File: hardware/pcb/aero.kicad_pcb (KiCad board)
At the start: 4 copper layers, 39.1 x 46.2 mm, 91 parts, among them CON1 USB-MICRO-B, CON2 MMCX_CONN, J1 CORTEX_DBG_CONN, J2 LiPoly_Conn, Q1 Q_NPN_BEC, SW1 SW_PUSH, U1 STM32L151C8, U2 nRF8001, U3 ms5611, U4 BMX055, U5 AT45DB321E, U6 BQ24040DSQ, U7 TPS783, U8 TPS61041, U9 ZXMHC6A07N8, Y1 Crystal, Y2 Crystal, Y3 32.768KHz, Y4 16MHz

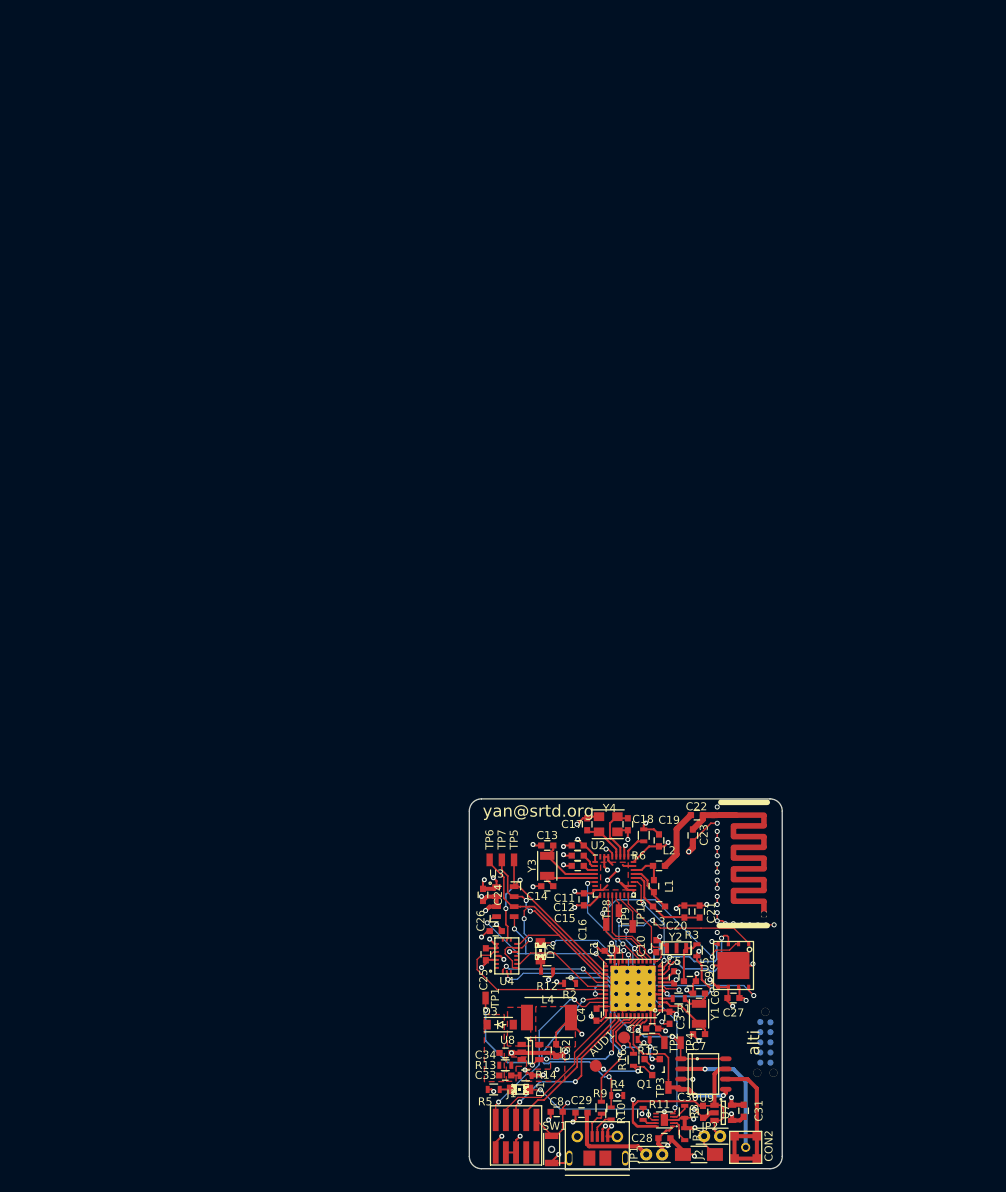
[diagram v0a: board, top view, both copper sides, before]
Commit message: more progress on new layout
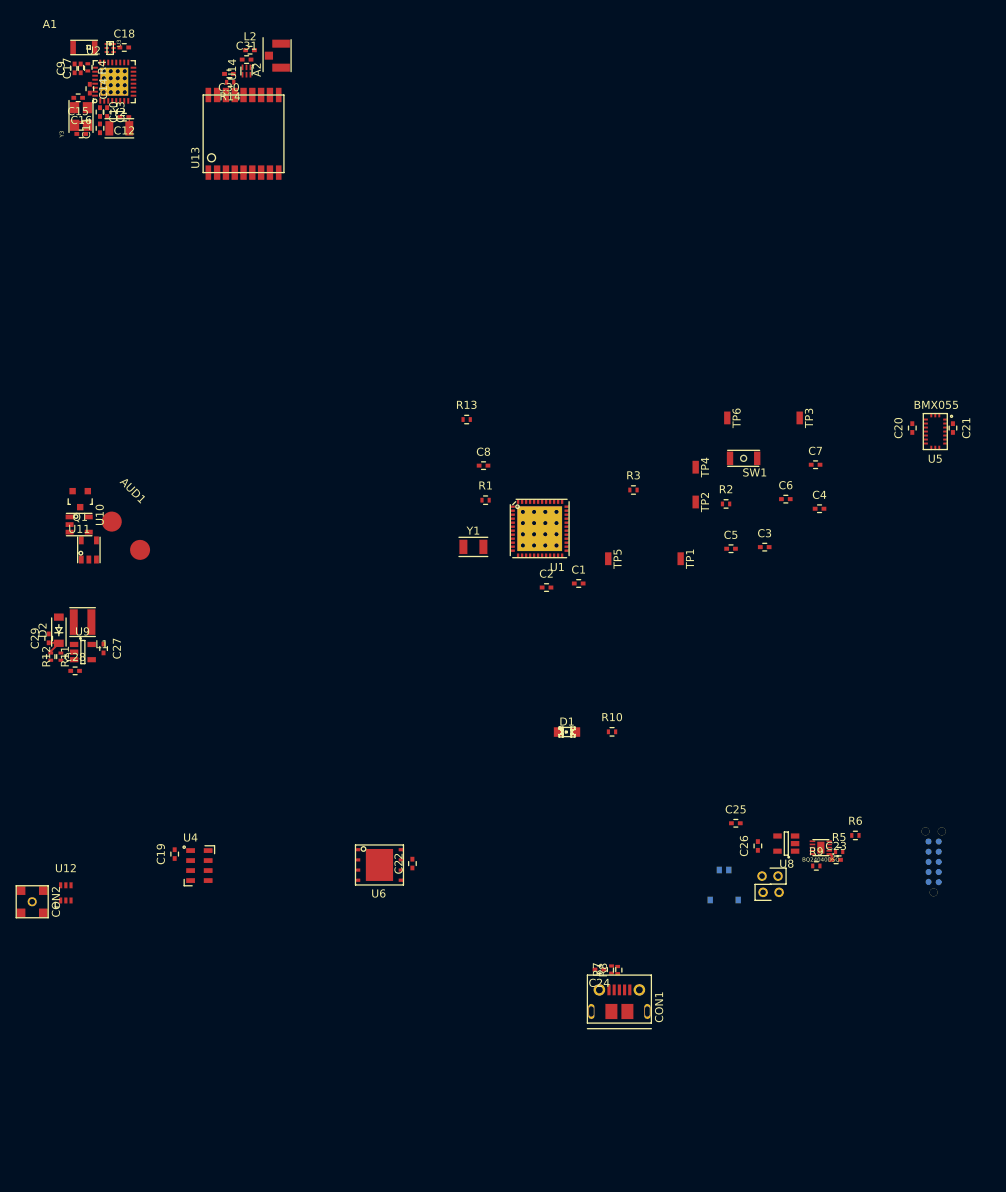
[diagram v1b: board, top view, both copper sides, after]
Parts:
- removed Ant_Bluetooth: VAL**, aero:Ant_Bluetooth
- removed C32: 4.7uF, Capacitors_SMD:C_0603
- removed C33: 22pF, Capacitors_SMD:C_0603
- removed C34: 100nF, Capacitors_SMD:C_0603
- removed D3: D_Schottky, Diodes_SMD:SOD-123
- removed L3: 5.6nH, Capacitors_SMD:C_0603
- removed L4: 10u, aero:SDR0703
- removed R15: 3k, Resistors_SMD:R_0603
- removed R16: 2k, Resistors_SMD:R_0603
- removed REF**: TC2050-IDC-NL, aero:TC2050-IDC-NL
- removed TP10, TP7, TP8, TP9: Test_Point, aero:TP_0603
- removed Y4: 16MHz, aero:crystal_SMD_3225
- added A1: 2450AT18A100, aero:2450AT18A100, F.Cu at (112.3, 17.8)
- added A2: U.FL_Antenna, aero:U.FL, F.Cu at (137.0, 18.9)
- added U10: BU4SU69G2, aero:SSOP-5, F.Cu at (111.8, 77.5)
- added U11: BU4SU69G2, aero:SSOP-5, F.Cu at (113.0, 80.6)
- added U12: NC7WZ17, Housings_SOT-23_SOT-143_TSOT-6:SC-70-6, F.Cu at (110.1, 123.5)
- added U13: u-blox_max-7c/q, aero:ublox_MAX7, F.Cu at (132.3, 28.6)
- added U14: MAX2659, aero:6-µDFN, F.Cu at (132.7, 20.8)
- C1, C2, C3, C4, C5, C6, C7, C8: footprint Capacitors_SMD:C_0603 -> Capacitors_SMD:C_0402
- C10, C14, C9: value 15pF -> 100nF; footprint Capacitors_SMD:C_0603 -> Capacitors_SMD:C_0402
- C11, C12: value 100nF -> 15pF; footprint Capacitors_SMD:C_0603 -> Capacitors_SMD:C_0402
- C13: value 15pF -> 33nF; footprint Capacitors_SMD:C_0603 -> Capacitors_SMD:C_0402
- C15: value 33nF -> 12pF; footprint Capacitors_SMD:C_0603 -> Capacitors_SMD:C_0402
- C16: value 100nF -> 12pF; footprint Capacitors_SMD:C_0603 -> Capacitors_SMD:C_0402
- C17: value 12pF -> 1.0nF; footprint Capacitors_SMD:C_0603 -> Capacitors_SMD:C_0402
- C18: value 12pF -> 2.2nF; footprint Capacitors_SMD:C_0603 -> Capacitors_SMD:C_0402
- C19: value 1.0nF -> 100nF; footprint Capacitors_SMD:C_0603 -> Capacitors_SMD:C_0402
- C20: value 2.2nF -> 100nF; footprint Capacitors_SMD:C_0603 -> Capacitors_SMD:C_0402
- C21: value NC -> 100nF; footprint Capacitors_SMD:C_0603 -> Capacitors_SMD:C_0402
- C22: value 1.8pF -> 100nF; footprint Capacitors_SMD:C_0603 -> Capacitors_SMD:C_0402
- C23: value 1.2pF -> 1uF; footprint Capacitors_SMD:C_0603 -> Capacitors_SMD:C_0402
- C24, C25: value 100nF -> 1uF; footprint Capacitors_SMD:C_0603 -> Capacitors_SMD:C_0402
- C26: value 100nF -> 2.2uF; footprint Capacitors_SMD:C_0603 -> Capacitors_SMD:C_0402
- C27: value 100nF -> 4.7uF; footprint Capacitors_SMD:C_0603 -> Capacitors_SMD:C_0402
- C28: value 1uF -> 22pF; footprint Capacitors_SMD:C_0603 -> Capacitors_SMD:C_0402
- C29: value 1uF -> 100nF; footprint Capacitors_SMD:C_0603 -> Capacitors_SMD:C_0402
- C30: value 1uF -> 33nF; footprint Capacitors_SMD:C_0603 -> Capacitors_SMD:C_0402
- C31: value 2.2uF -> 470pF; footprint Capacitors_SMD:C_0603 -> Capacitors_SMD:C_0402
- D2: value LED -> D_Schottky; footprint LEDs:LED-0805 -> Diodes_SMD:SOD-123
- J1: footprint aero:FTSH-105-01 -> aero:TC2050-IDC-NL; moved to B.Cu
- J2: footprint Capacitors_SMD:C_1206_HandSoldering -> aero:Conn_Molex_78171-02; moved to B.Cu
- JP1, JP2: footprint aero:Pin_Header_1x02 -> aero:Pin_Header_1x02_2mm
- L1: value 8.2nH -> 10u; footprint Capacitors_SMD:C_0603 -> aero:IND-744029100
- L2: value 3.9nH -> 6.8nH; footprint Capacitors_SMD:C_0603 -> Capacitors_SMD:C_0402
- Q1: value Q_NPN_BEC -> BSS138
- R1, R2: footprint Resistors_SMD:R_0603 -> Resistors_SMD:R_0402
- R10: value 22 -> 200; footprint Resistors_SMD:R_0603 -> Resistors_SMD:R_0402
- R11: value 10k -> 2.21m; footprint Resistors_SMD:R_0603 -> Resistors_SMD:R_0402
- R12: value 120 -> 309k; footprint Resistors_SMD:R_0603 -> Resistors_SMD:R_0402
- R13: value 2.21m -> 30k; footprint Resistors_SMD:R_0603 -> Resistors_SMD:R_0402
- R14: value 140k -> 10k; footprint Resistors_SMD:R_0603 -> Resistors_SMD:R_0402
- R3: value 220 -> 1.5k; footprint Resistors_SMD:R_0603 -> Resistors_SMD:R_0402
- R4: value 1.5k -> 22k; footprint Resistors_SMD:R_0603 -> Resistors_SMD:R_0402
- R5: value 1.5k -> 825; footprint Resistors_SMD:R_0603 -> Resistors_SMD:R_0402
- R6: value 22k -> 2k; footprint Resistors_SMD:R_0603 -> Resistors_SMD:R_0402
- R7: value 825 -> 22; footprint Resistors_SMD:R_0603 -> Resistors_SMD:R_0402
- R8: value 2k -> 22; footprint Resistors_SMD:R_0603 -> Resistors_SMD:R_0402
- R9: value 22 -> 10k; footprint Resistors_SMD:R_0603 -> Resistors_SMD:R_0402
- U2: footprint Housings_DFN_QFN:QFN-32-1EP_5x5mm_Pitch0.5mm -> aero:QFN-32-1EP_5x5mm_Pitch0.5mm
- U3: value ms5611 -> 2450BM14A0002; footprint aero:ms5611 -> aero:2450BM14A0002
- U4: value BMX055 -> ms5611; footprint aero:BMX055 -> aero:ms5611
- U5: value AT45DB321E -> BMX055; footprint aero:UDFN-8 -> aero:BMX055
- U6: value BQ24040DSQ -> AT45DB321E; footprint aero:WSON-10-1EP -> aero:UDFN-8
- U7: value TPS783 -> BQ24040DSQ; footprint Housings_SOT-23_SOT-143_TSOT-6:SOT-23-5 -> aero:WSON-10-1EP
- U8: value TPS61041 -> TPS783
- U9: value ZXMHC6A07N8 -> TPS61041; footprint Power_Integrations:SO-8 -> Housings_SOT-23_SOT-143_TSOT-6:SOT-23-5
- Y1: footprint aero:FC-135R -> aero:Crystal_32768_FC-135R
- Y2: value Crystal -> 32.768KHz; footprint aero:Murata_CSTCE-G_Oscillator -> aero:Crystal_32768_FC-135R
- Y3: value 32.768KHz -> 16MHz; footprint aero:FC-135R -> aero:Crystal_TSX_3225
- moved C31 145.3 mm to (132.7, 19.3), turned to 0 degrees
- moved R4 144.6 mm to (112.8, 20.3), turned to 270 degrees
- moved C30 142.6 mm to (130.5, 21.1), turned to 180 degrees
- moved C9 137.6 mm to (111.2, 20.4), turned to 90 degrees
- moved R14 129.5 mm to (130.6, 22.2), turned to 180 degrees
- moved C10 125.3 mm to (114.4, 25.9), turned to 270 degrees
- moved Y2 123.9 mm to (116.8, 27.9), turned to 0 degrees
- moved U3 117.6 mm to (115.6, 17.9), turned to 90 degrees
- moved U2 117.3 mm to (116.1, 22.1), turned to 90 degrees
- moved C18 115.7 mm to (117.4, 17.8), turned to 0 degrees
- moved C14 114.9 mm to (113.1, 23.0), turned to 270 degrees
- moved C15 114.5 mm to (111.6, 24.1)
- moved C16 114.5 mm to (112.0, 28.6), turned to 0 degrees
- moved L2 114.1 mm to (133.1, 18.2)
- moved C17 113.7 mm to (112.0, 20.4), turned to 90 degrees
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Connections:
- C1 pad 1: +3V3 -> +3V
- C10 pad 1: GND -> Net-(C10-Pad1)
- C10 pad 2: Net-(C10-Pad2) -> GND
- C11 pad 1: +3V3 -> Net-(C11-Pad1)
- C14 pad 1: Net-(C14-Pad1) -> +3V
- C15 pad 1: Net-(C15-Pad1) -> GND
- C15 pad 2: GND -> Net-(C15-Pad2)
- C16 pad 1: +3V3 -> GND
- C16 pad 2: GND -> Net-(C16-Pad2)
- C17 pad 1: GND -> +3V
- C17 pad 2: Net-(C17-Pad2) -> GND
- C18 pad 1: GND -> Net-(C18-Pad1)
- C18 pad 2: Net-(C18-Pad2) -> GND
- C19 pad 1: +3V3 -> +3V
- C2 pad 1: +3V3 -> +3V
- C20 pad 1: Net-(C20-Pad1) -> +3V
- C21 pad 1: Net-(C20-Pad1) -> +3V
- C22 pad 1: /nRF8001/Antenna -> +3V
- C22 pad 2: Net-(C22-Pad2) -> GND
- C23 pad 1: /nRF8001/Antenna -> Net-(C23-Pad1)
- C24 pad 1: +3V3 -> Net-(C24-Pad1)
- C25 pad 1: +3V3 -> Vbatt
- C26 pad 1: +3V3 -> +3V
- C27 pad 1: +3V3 -> Vbatt
- C28 pad 1: Net-(C28-Pad1) -> +10V
- C28 pad 2: GND -> Net-(C28-Pad2)
- C29 pad 1: Net-(C29-Pad1) -> +10V
- C3 pad 1: +3V3 -> +3V
- C30 pad 1: Vbatt -> Net-(C30-Pad1)
- C31 pad 1: +3V3 -> Net-(C31-Pad1)
- C31 pad 2: GND -> Net-(C31-Pad2)
- C4 pad 1: +3V3 -> +3V
- C5 pad 1: +3V3 -> +3V
- C9 pad 1: Net-(C9-Pad1) -> +3V
- CON1 pad 1: Net-(C29-Pad1) -> Net-(C24-Pad1)
- CON2 pad 1: Net-(CON2-Pad2) -> Net-(CON2-Pad1)
- CON2 pad 2: Net-(CON2-Pad1) -> Net-(CON2-Pad2)
- D1 pad 2: /power/~CHG -> /warn/STATUS_LED
- D2 pad 1: /warn/STATUS_LED -> +10V
- J1 pad 1: +3V3 -> +3V
- JP1 pad 1: Net-(C29-Pad1) -> Net-(C24-Pad1)
- JP1 pad 2: Net-(C28-Pad1) -> Net-(C23-Pad1)
- L1 pad 1: Net-(L1-Pad1) -> Net-(D2-Pad2)
- L1 pad 2: Net-(L1-Pad2) -> Vbatt
- L2 pad 1: Net-(L1-Pad2) -> Net-(C31-Pad2)
- L2 pad 2: Net-(C22-Pad2) -> Net-(A2-Pad1)
- Q1 pad 1: Net-(Q1-Pad1) -> /warn/PIEZO_OUT
- Q1 pad 3: Net-(AUD1-Pad2) -> Net-(Q1-Pad3)
- R10 pad 1: /power/USB_D+ -> GND
- R10 pad 2: Net-(CON1-Pad3) -> Net-(D1-Pad1)
- R11 pad 1: GND -> +10V
- R11 pad 2: Net-(R11-Pad2) -> Net-(C28-Pad2)
- R12 pad 1: GND -> Net-(C28-Pad2)
- R12 pad 2: Net-(D2-Pad2) -> GND
- R13 pad 1: Net-(C33-Pad1) -> +10V
- R13 pad 2: Net-(C33-Pad2) -> Net-(Q1-Pad3)
- R14 pad 1: Net-(C33-Pad2) -> Net-(R14-Pad1)
- R3 pad 1: Net-(C9-Pad1) -> +3V
- R3 pad 2: Net-(R3-Pad2) -> /power/USB_D+
- R4 pad 1: +3V3 -> GND
- R4 pad 2: /power/USB_D+ -> Net-(R4-Pad2)
- R5 pad 1: GND -> Net-(R5-Pad1)
- R5 pad 2: Net-(D1-Pad1) -> GND
- R6 pad 1: GND -> Net-(R6-Pad1)
- R6 pad 2: Net-(R6-Pad2) -> GND
- R7 pad 1: Net-(R7-Pad1) -> /power/USB_D-
- R7 pad 2: GND -> Net-(CON1-Pad2)
- R8 pad 1: Net-(R8-Pad1) -> /power/USB_D+
- R8 pad 2: GND -> Net-(CON1-Pad3)
- R9 pad 1: /power/USB_D- -> GND
- R9 pad 2: Net-(CON1-Pad2) -> Net-(R9-Pad2)
- TP1 pad 1: /warn/PIEZO_EN -> /bmx055/SCK
- TP2 pad 1: /warn/PIEZO_OUT -> /bmx055/MISO
- TP3 pad 1: /warn/WARN_LED_A -> /bmx055/MOSI
- TP4 pad 1: /warn/WARN_LED_B -> /at45db321e/SCK
- TP5 pad 1: /bmx055/SCK -> /at45db321e/MOSI
- TP6 pad 1: /bmx055/MISO -> /at45db321e/MISO
- U1 pad 1: +3V3 -> +3V
- U1 pad 18: Net-(U1-Pad18) -> /bmx055/ACC_SEL
- U1 pad 19: ~PG -> /bmx055/GYRO_SEL
- U1 pad 2: Net-(U1-Pad2) -> /GPS/TIMEPULSE
- U1 pad 20: Net-(U1-Pad20) -> /bmx055/MAG_SEL
- U1 pad 24: +3V3 -> +3V
- U1 pad 29: MAG_SEL -> Net-(U1-Pad29)
- U1 pad 30: ACC_SEL -> ~PG
- U1 pad 31: GYRO_SEL -> ~CHG
- U1 pad 36: +3V3 -> +3V
- U1 pad 40: ACC_INT -> /warn/PIEZO_EN
- U1 pad 41: Net-(U1-Pad41) -> /warn/PIEZO_OUT
- U1 pad 42: /warn/PIEZO_EN -> /GPS/RxD
- U1 pad 43: /warn/PIEZO_OUT -> /GPS/TxD
- U1 pad 48: +3V3 -> +3V
- U1 pad 49: GND -> (no net)
- U1 pad 5: Net-(C10-Pad2) -> /GPS/RESET
- U1 pad 6: Net-(R3-Pad2) -> /GPS/EXT_INT
- U1 pad 9: +3V3 -> +3V
- U2 pad 1: +3V3 -> +3V
- U2 pad 2: Net-(C12-Pad1) -> Net-(C10-Pad1)
- U2 pad 20: Net-(C20-Pad1) -> Net-(C18-Pad1)
- U2 pad 21: Net-(L1-Pad1) -> Net-(U2-Pad21)
- U2 pad 22: Net-(L1-Pad2) -> Net-(U2-Pad22)
- U2 pad 24: +3V3 -> +3V
- U2 pad 25: Net-(R6-Pad2) -> Net-(R4-Pad2)
- U2 pad 26: +3V3 -> +3V
- U2 pad 27: Net-(C18-Pad2) -> Net-(C16-Pad2)
- U2 pad 28: Net-(C17-Pad2) -> Net-(C15-Pad2)
- U2 pad 29: +3V3 -> +3V
- U2 pad 3: Net-(C15-Pad1) -> Net-(C13-Pad1)
- U2 pad 4: Net-(C13-Pad1) -> Net-(C11-Pad1)
- U2 pad 5: Net-(C14-Pad1) -> Net-(C12-Pad1)
- U2 pad 9: +3V3 -> +3V
- U3 pad 1: +3V3 -> Net-(A1-Pad1)
- U3 pad 3: GND -> Net-(U2-Pad22)
- U3 pad 4: /ms5611/EN -> Net-(U2-Pad21)
- U3 pad 5: /ms5611/EN -> Net-(C18-Pad1)
- U3 pad 6: /bmx055/MISO -> Net-(U3-Pad6)
- U4 pad 1: Net-(U4-Pad1) -> +3V
- U4 pad 2: Net-(U4-Pad2) -> GND
- U4 pad 3: +3V3 -> GND
- U4 pad 4: GND -> /ms5611/EN
- U4 pad 5: GYRO_SEL -> /ms5611/EN
- U4 pad 6: GND -> /bmx055/MISO
- U4 pad 7: GND -> /bmx055/MOSI
- U4 pad 8: Net-(U4-Pad8) -> /bmx055/SCK
- U5 pad 1: /at45db321e/MOSI -> Net-(U5-Pad1)
- U5 pad 2: /at45db321e/SCK -> Net-(U5-Pad2)
- U5 pad 3: /at45db321e/~RESET -> +3V
- U5 pad 4: /at45db321e/~CS -> GND
- U5 pad 5: +3V3 -> /bmx055/GYRO_SEL
- U5 pad 6: +3V3 -> GND
- U5 pad 8: /at45db321e/MISO -> Net-(U5-Pad8)
- U6 pad 1: Net-(C28-Pad1) -> /at45db321e/MOSI
- U6 pad 2: Net-(R7-Pad1) -> /at45db321e/SCK
- U6 pad 3: GND -> /at45db321e/~RESET
- U6 pad 4: Net-(R8-Pad1) -> /at45db321e/~CS
- U6 pad 5: ~PG -> +3V
- U6 pad 6: Net-(U6-Pad6) -> +3V
- U6 pad 7: Net-(U6-Pad7) -> GND
- U6 pad 8: /power/~CHG -> /at45db321e/MISO
- U7 pad 1: Vbatt -> Net-(C23-Pad1)
- U7 pad 2: GND -> Net-(R5-Pad1)
- U7 pad 3: Vbatt -> GND
- U7 pad 4: GND -> Net-(R6-Pad1)
- U7 pad 5: +3V3 -> ~PG
- U8 pad 1: Net-(D3-Pad2) -> Vbatt
- U8 pad 3: Net-(C33-Pad2) -> Vbatt
- U8 pad 4: /warn/PIEZO_EN -> GND
- U8 pad 5: Vbatt -> +3V
- U9 pad 1: /warn/WARN_LED_B -> Net-(D2-Pad2)
- U9 pad 2: Net-(CON2-Pad1) -> GND
- U9 pad 3: GND -> Net-(C28-Pad2)
- U9 pad 4: /warn/WARN_LED_A -> /warn/PIEZO_EN
- U9 pad 5: /warn/WARN_LED_A -> Vbatt
- Y2 pad 1: Net-(C9-Pad1) -> Net-(C11-Pad1)
- Y2 pad 2: Net-(C10-Pad2) -> Net-(C12-Pad1)
- Y3 pad 1: Net-(C13-Pad1) -> Net-(C15-Pad2)
- Y3 pad 2: Net-(C14-Pad1) -> Net-(C16-Pad2)
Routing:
- net GND: track 288.5 -> 0.00 mm, vias 86 -> 0
- net Vbatt: track 50.8 -> 0.00 mm, vias 2 -> 0
- net +3V3: track 49.4 -> 0.00 mm, vias 20 -> 0
- net /at45db321e/SCK: track 34.9 -> 0.00 mm, vias 2 -> 0
- net /bmx055/MISO: track 33.9 -> 0.00 mm, vias 2 -> 0
- net ~NRST: track 32.3 -> 0.00 mm, vias 2 -> 0
- net /warn/PIEZO_EN: track 29.1 -> 0.00 mm, vias 4 -> 0
- net /bmx055/SCK: track 28.6 -> 0.00 mm, vias 2 -> 0
- net /bmx055/MOSI: track 27.3 -> 0.00 mm, vias 2 -> 0
- net /at45db321e/MOSI: track 27.3 -> 0.00 mm, vias 3 -> 0
- net /power/USB_D+: track 25.6 -> 0.00 mm, vias 2 -> 0
- net Net-(J1-Pad2): track 25.2 -> 0.00 mm, vias 2 -> 0
- net /ms5611/EN: track 24.0 -> 0.00 mm, vias 3 -> 0
- net Net-(CON2-Pad2): track 21.5 -> 0.00 mm
- net GYRO_SEL: track 21.3 -> 0.00 mm
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- removed copper zone on In2.Cu, net +3V3
- removed copper zone on F.Cu, net GND
- removed copper zone on In1.Cu, net GND
- removed copper zone on F.Cu, net Net-(C33-Pad1)
- removed copper zone on F.Cu, net Net-(C33-Pad2)
- removed copper zone on F.Cu, net Net-(D3-Pad2)
- removed copper zone on F.Cu, net Vbatt
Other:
- board outline removed
- net class Default: clearance 0.1524 -> 0.2; trace_width 0.1524 -> 0.25; via_dia 0.635 -> 0.6; via_drill 0.381 -> 0.4
- rule trace_clearance: 0.1524 -> 0.2
- rule via_min_drill: 0.381 -> 0.254
- rule via_min_size: 0.635 -> 0.3556
- board text removed: "alti"
- board text removed: "yan@srtd.org"

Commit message: more pcb rework
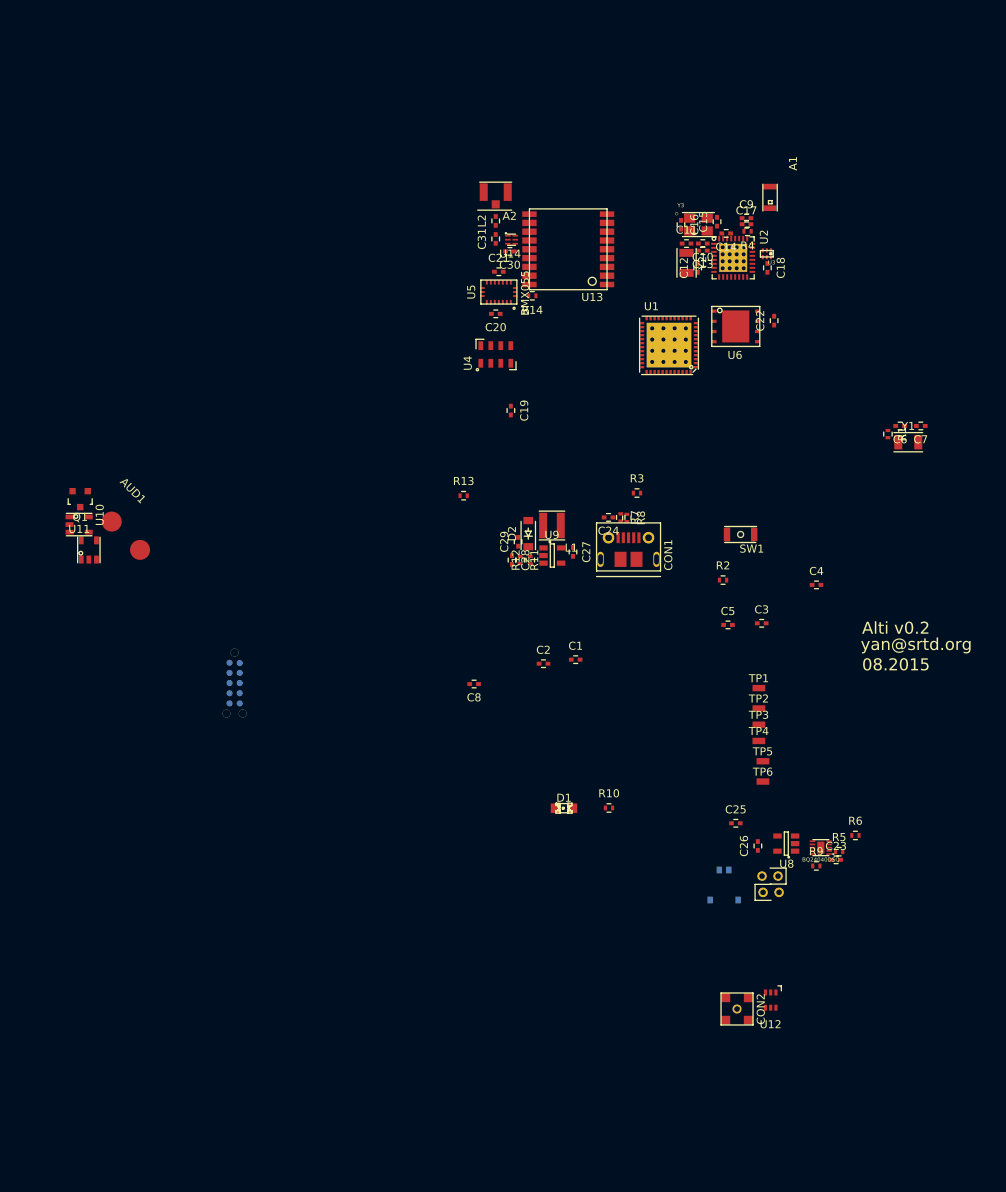
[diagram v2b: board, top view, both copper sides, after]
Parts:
- added REF**: v, aero:Via_Stitch, F.Cu at (186.4, 38.6)
- moved J1 90.2 mm to (131.2, 97.3), turned to 270 degrees
- moved U12 89.1 mm to (198.2, 136.9), turned to 180 degrees
- moved CON2 89.1 mm to (194.0, 138.0)
- moved A1 87.8 mm to (198.1, 36.6), turned to 90 degrees
- moved C9 86.0 mm to (195.2, 39.2), turned to 0 degrees
- moved U3 86.0 mm to (197.7, 43.6), turned to 0 degrees
- moved C17 85.5 mm to (195.2, 39.9), turned to 0 degrees
- moved C18 85.0 mm to (197.8, 45.4), turned to 270 degrees
- moved R4 85.0 mm to (195.3, 40.8), turned to 180 degrees
- moved C14 81.6 mm to (192.6, 41.1), turned to 180 degrees
- moved C22 81.5 mm to (198.6, 52.0)
- moved C15 81.3 mm to (191.5, 39.6), turned to 90 degrees
- moved U6 80.7 mm to (193.8, 52.7)
- moved U2 80.4 mm to (193.5, 44.1), turned to 0 degrees
- moved Y3 78.3 mm to (189.2, 40.0), turned to 180 degrees
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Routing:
- net +10V: track 2.94 -> 0.00 mm
- net Net-(C12-Pad1): track 1.42 -> 0.00 mm
- net (no net): track 1.42 -> 0.00 mm
- net Net-(C23-Pad1): track 0.89 -> 0.00 mm
- net Net-(R14-Pad1): track 0.68 -> 0.00 mm
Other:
- board text added: "08.2015"
- board text added: "Alti v0.2"
- board text added: "yan@srtd.org"
